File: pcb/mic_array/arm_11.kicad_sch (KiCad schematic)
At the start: 16 parts, among them U89 IM72D128V01XTMA1, U90 IM72D128V01XTMA1, U91 IM72D128V01XTMA1, U92 IM72D128V01XTMA1, U93 IM72D128V01XTMA1, U94 IM72D128V01XTMA1, U95 IM72D128V01XTMA1, U96 IM72D128V01XTMA1

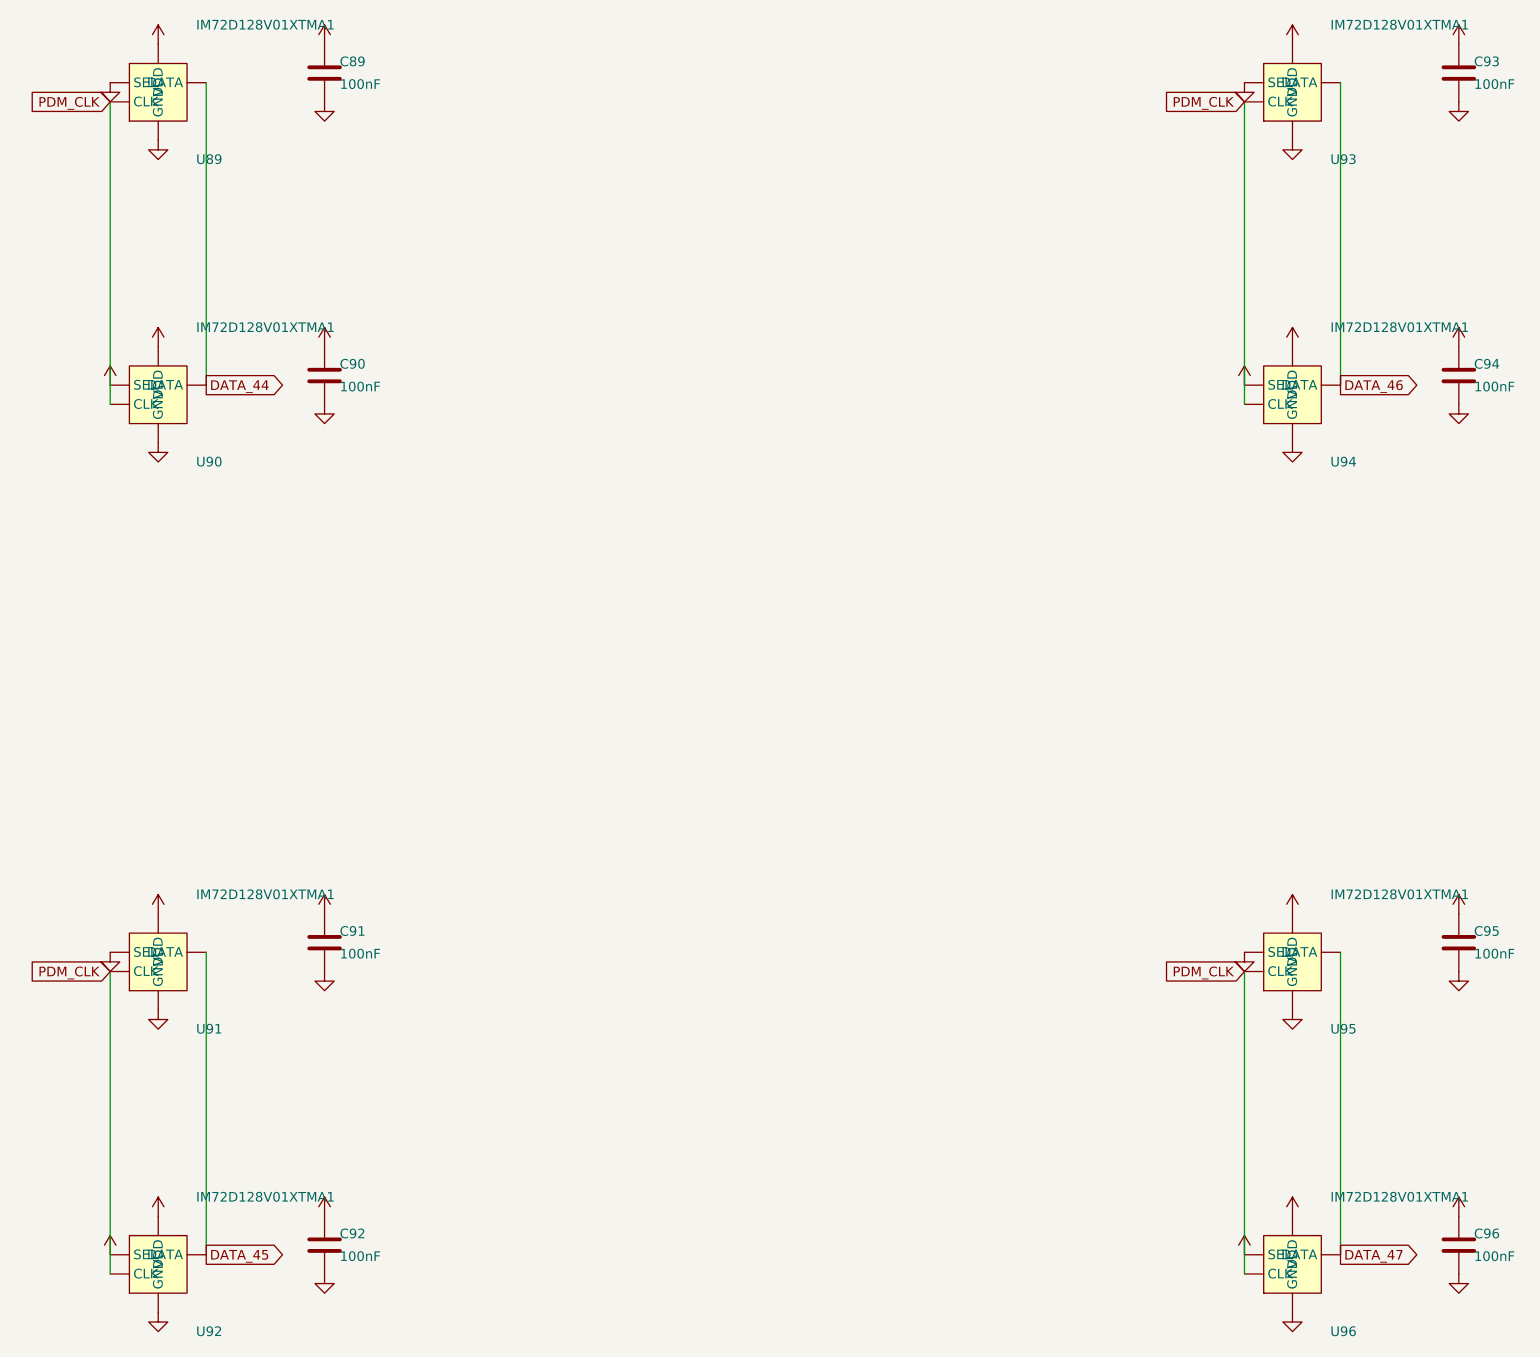
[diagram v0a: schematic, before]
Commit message: Updated.
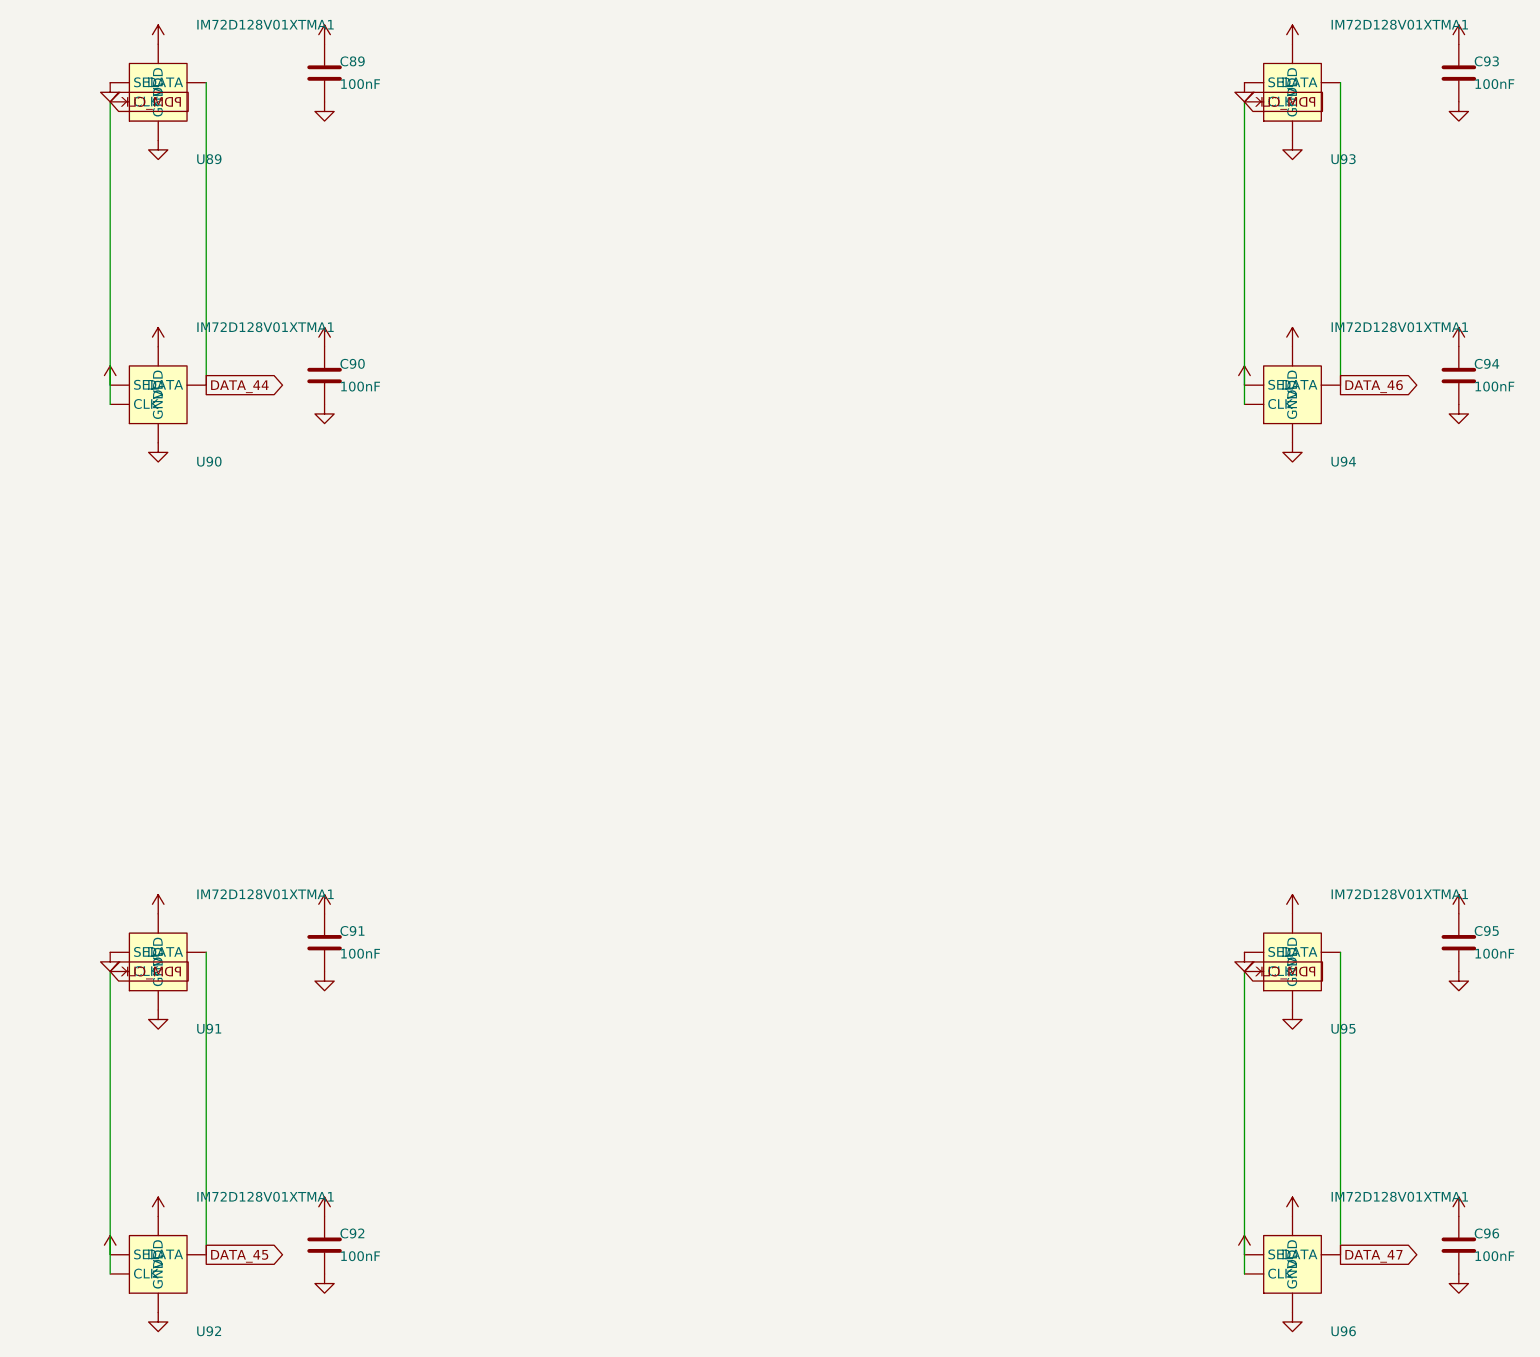
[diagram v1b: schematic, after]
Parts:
- C89, C90, C91, C92, C93, C94, C95, C96: footprint Capacitor_SMD:C_0402_1005Metric -> (none)
- U89, U90, U91, U92, U93, U94, U95, U96: footprint Sensor_Audio:Infineon_PG-LLGA-5-2 -> (none)
